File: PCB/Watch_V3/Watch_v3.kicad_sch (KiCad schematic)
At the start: 85 parts, among them J1 USB_C_Receptacle_USB2.0_16P, J2 Screw_Terminal, J3 Peripheral, J4 OLED, J5 BN220, J6 Peripheral, J7 MAX30102, M1 Motor_DC, Q1 AO3401A, Q2 BC817, Q3 BC817, Q4 SI2302, Q5 BC847, SW1 SW_DPST_x2, SW2 SW_SPDT, SW3 SW_DPST_x2, SW4 Select, SW5 Mode, SW6 Up, SW7 Down, U1 AP2112K-3.3, U2 AP2112K-3.3, U3 TP4056, U4 ESP32-WROOM-32D, U5 CH340G, U6 MPU-6050, Y1 12M

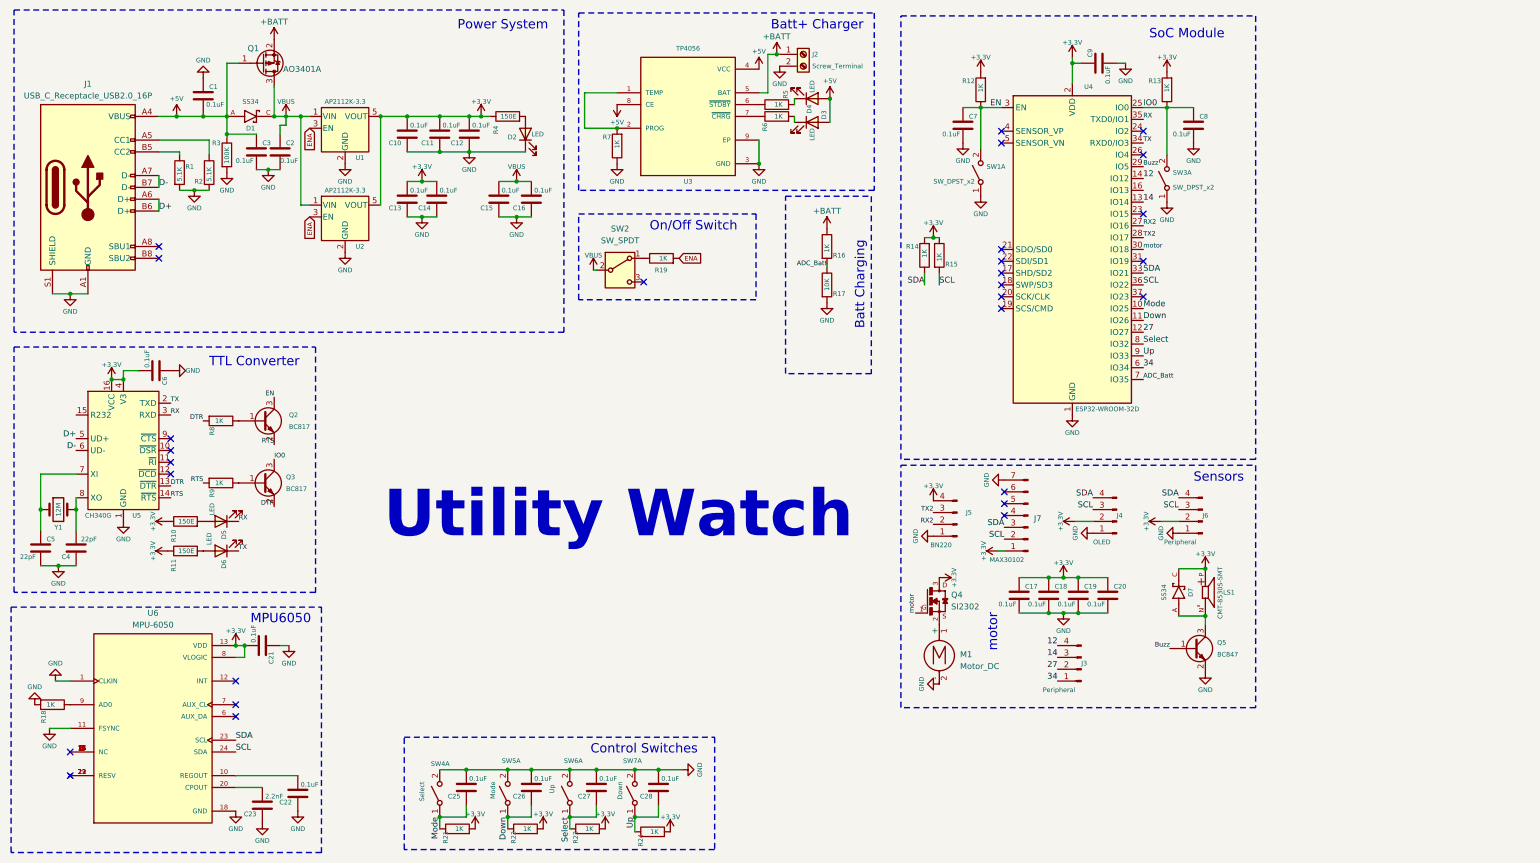
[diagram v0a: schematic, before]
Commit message: updating watchV3
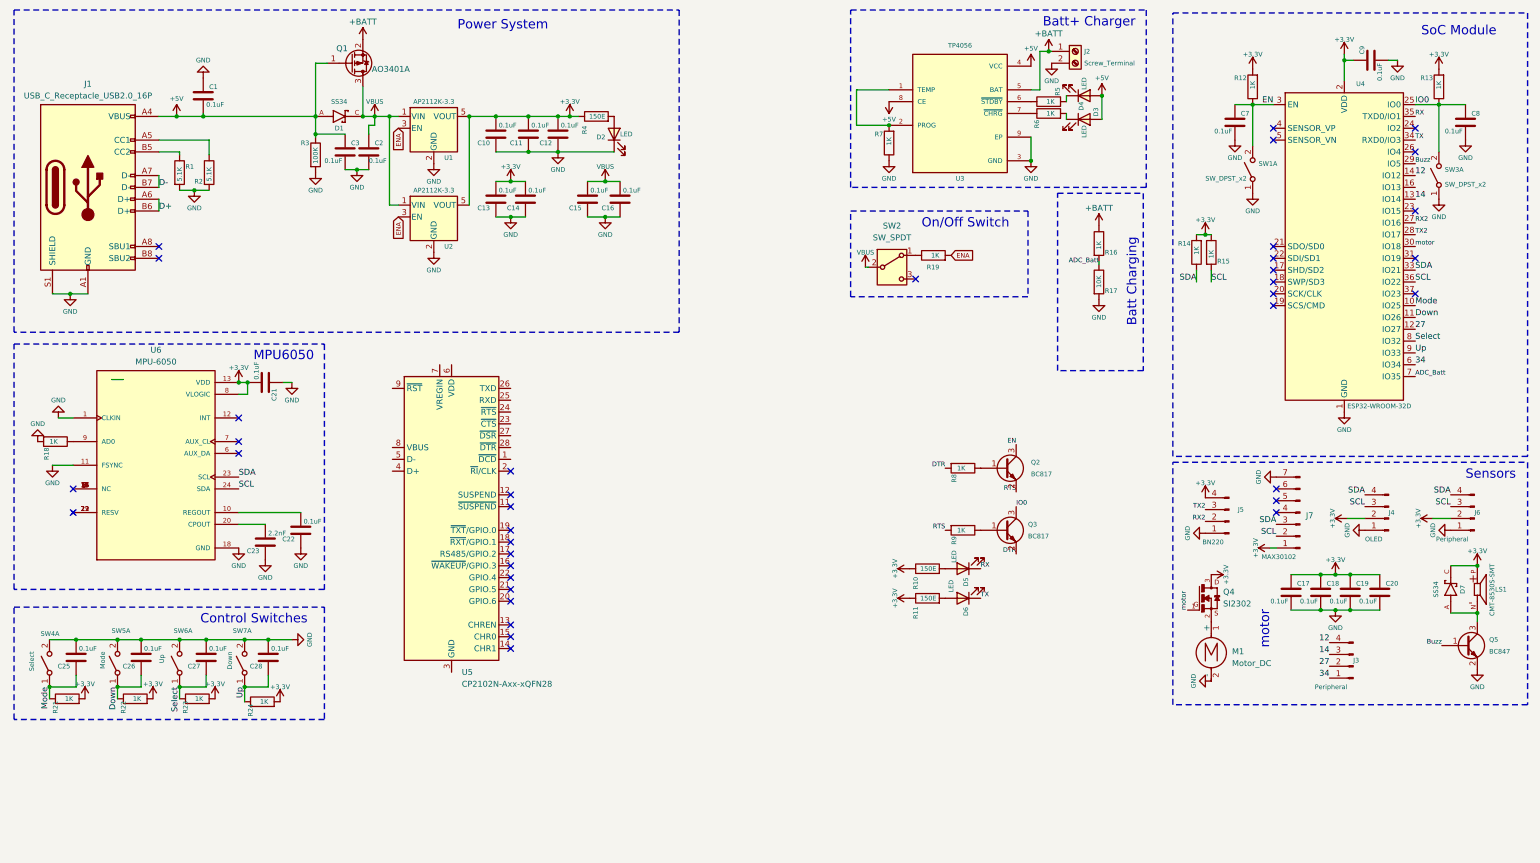
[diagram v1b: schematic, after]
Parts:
- removed C4, C5: 22pF, Capacitor_SMD:C_0402_1005Metric, symbol Device:C
- removed C6: 0.1uF, Capacitor_SMD:C_0402_1005Metric, symbol Device:C
- removed U5: CH340G, Package_SO:SOIC-16_3.9x9.9mm_P1.27mm, symbol Interface_USB:CH340G
- removed Y1: 12M, Crystal:Crystal_HC49-4H_Vertical, symbol Device:Crystal
- added U5: CP2102N-Axx-xQFN28, Package_DFN_QFN:QFN-28-1EP_5x5mm_P0.5mm_EP3.35x3.35mm, symbol Interface_USB:CP2102N-Axx-xQFN28
- SW4, SW5, SW6, SW7: footprint Button_Switch_SMD:SW_Push_1P1T_NO_6x6mm_H9.5mm -> Button_Switch_SMD:SW_Tactile_SPST_NO_Straight_CK_PTS636Sx25SMTRLFS
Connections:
- new net: U5.29 (GND), U5.3 (GND)
- no-connect marks 28 -> 37
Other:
- note removed: "TTL Converter"
- note removed: "Utility Watch"
- moved on the sheet: C10, C11, C12, C13, C14, C15, C16, C17, C18, C19, C2, C20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

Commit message: updating watch_V3
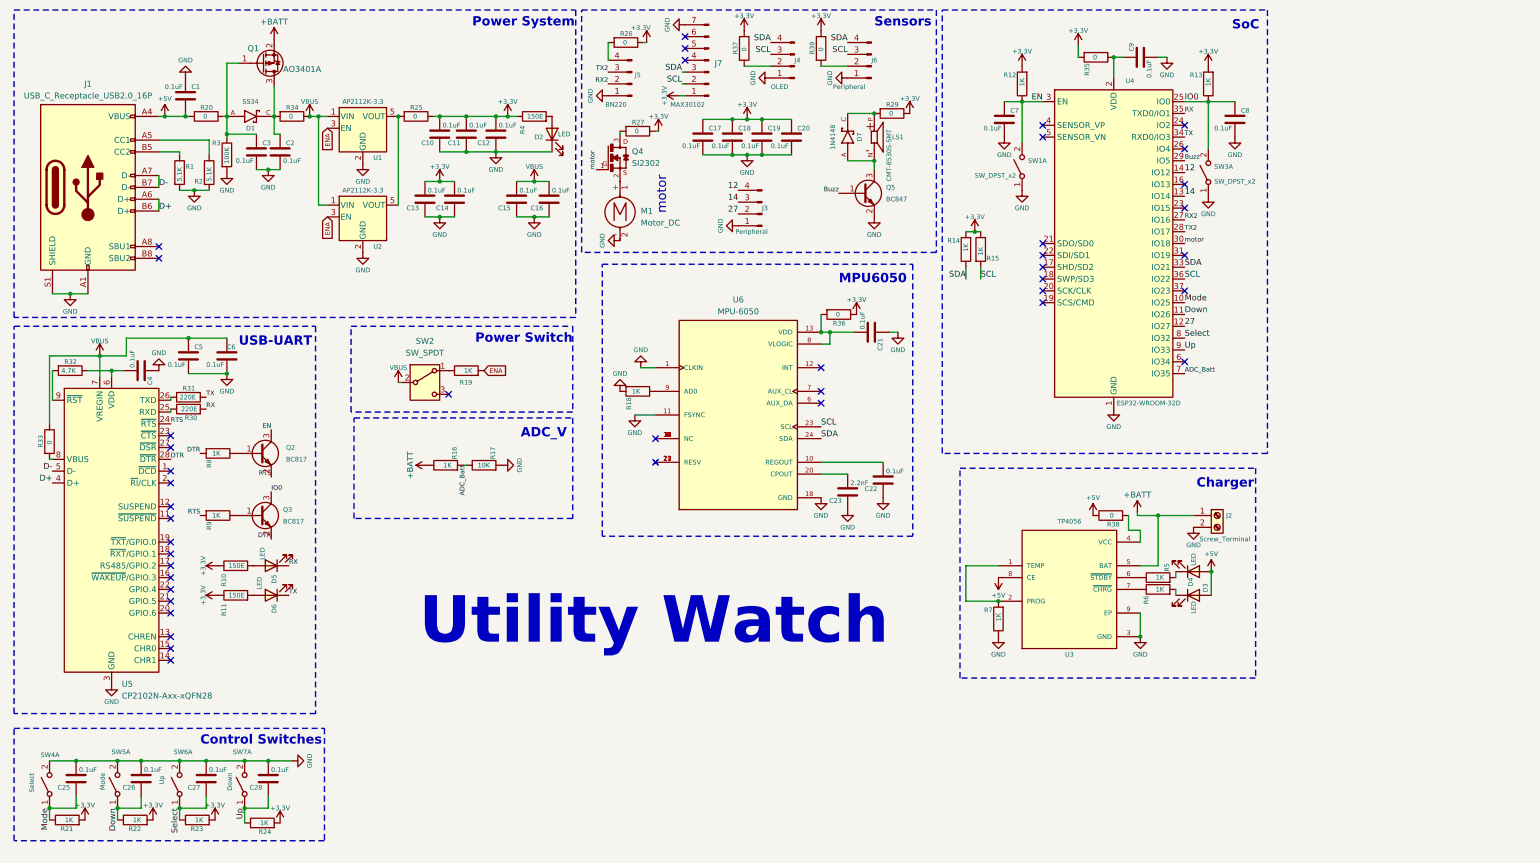
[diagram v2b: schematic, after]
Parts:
- added C4, C5, C6: 0.1uF, Capacitor_SMD:C_0402_1005Metric, symbol Device:C
- added R20, R25, R26, R27, R29, R33, R34, R35, R36, R37, R38, R39: 0, Resistor_SMD:R_0402_1005Metric, symbol Device:R
- added R30, R31: 220E, Resistor_SMD:R_0402_1005Metric, symbol Device:R
- added R32: 4.7K, Resistor_SMD:R_0402_1005Metric, symbol Device:R
- D1: footprint Capacitor_SMD:ss34_DO -> Button_Switch_SMD:P25_DO-214AC_SMA
- D7: value SS34 -> 1N4148; footprint Capacitor_SMD:ss34_DO -> Diode_SMD:D_SOD-323
- J1: footprint Connector_USB:USB_C_Receptacle_HCTL_HC-TYPE-C-16P-01A -> Connector_USB:USB_C_Receptacle_GCT_USB4105-xx-A_16P_TopMnt_Horizontal
- R1, R10, R11, R12, R13, R14, R15, R16, R17, R18, R19, R2, R21, R22, R23, R24, R3, R4, R5, R6, R7, R8, R9: footprint Resistor_SMD:R_01005_0402Metric -> Resistor_SMD:R_0402_1005Metric
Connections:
- net +3.3V: now also R25.1, R26.1, R27.1, R29.1, R35.2, R36.1, R37.1, R39.1; no longer C21.1, C9.2, D7.C, J4.2 (Pin_2), J5.4 (Pin_4), J6.2 (Pin_2), LS1.P, Q4.3, U1.5 (VOUT), U2.5 (VOUT), U4.2 (VDD), U6.13 (VDD), U6.8 (VLOGIC)
- net +5V: now also R20.2, R38.1; no longer C3.2, D1.A, Q1.1 (G), R3.1, U3.4 (VCC)
- net D+: now also U5.4 (D+)
- net D-: now also U5.5 (D-)
- net DTR: now also U5.28 (~{DTR})
- net GND: now also J3.1 (Pin_1), U5.29 (GND), U5.3 (GND), C4.2, C5.1, C6.1
- net RTS: now also U5.24 (~{RTS})
- net RX: now also R30.2
- net SCL: now also U6.23 (SCL); no longer U6.24 (SDA)
- net SDA: now also U6.24 (SDA); no longer U6.23 (SCL)
- net TX: now also R31.1
- net VBUS: now also U5.7 (VREGIN), C5.2, C6.2, R33.1, R34.1; no longer C2.2, D1.C, Q1.3 (D)
- net at U5.25 (RXD): now also R30.1
- net at U5.26 (TXD): now also R31.2
- net at U5.6 (VDD): now also C4.1, R32.1
- net at U5.8 (VBUS): now also R33.2
- net at U5.9 (~{RST}): now also R32.2
- net 34: no longer names the net of U4.6 (IO34)
- net 34: no longer J3.1 (Pin_1)
- new net: R38.2, U3.4 (VCC)
- new net: J5.4 (Pin_4), R26.2
- new net: R25.2, U1.5 (VOUT), U2.5 (VOUT)
- new net: J4.2 (Pin_2), R37.2
- new net: C9.2, R35.1, U4.2 (VDD)
- new net: C3.2, D1.A, Q1.1 (G), R20.1, R3.1
- new net: D7.C, LS1.P, R29.2
- new net: C2.2, D1.C, Q1.3 (D), R34.2
- new net: Q4.3, R27.2
- new net: C21.1, R36.2, U6.13 (VDD), U6.8 (VLOGIC)
- new net: J6.2 (Pin_2), R39.2
- no-connect marks 37 -> 42
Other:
- note added: "ADC_V"
- note added: "Charger"
- note added: "Power Switch"
- note added: "SoC"
- note added: "USB-UART"
- note added: "Utility Watch"
- note removed: "Batt Charging"
- note removed: "Batt+ Charger"
- note removed: "On/Off Switch"
- note removed: "SoC Module"
- moved on the sheet: C1, C10, C11, C12, C13, C14, C15, C16, C17, C18, C19, C2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
